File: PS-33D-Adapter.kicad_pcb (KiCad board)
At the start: 2 copper layers, 19.1 x 10.2 mm, 8 parts, among them J1 CONN_05, J2 Conn_02x04_Counter_Clockwise, Q1 MOSFET-NCH-BSS138, Q2 MOSFET-NCH-BSS138

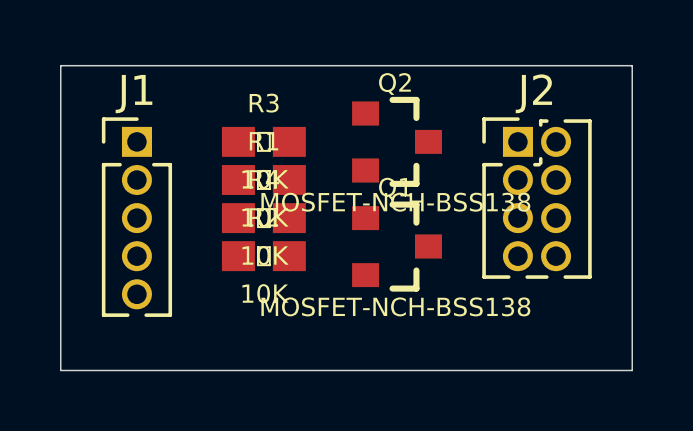
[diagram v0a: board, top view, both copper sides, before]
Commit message: feat: update pcb
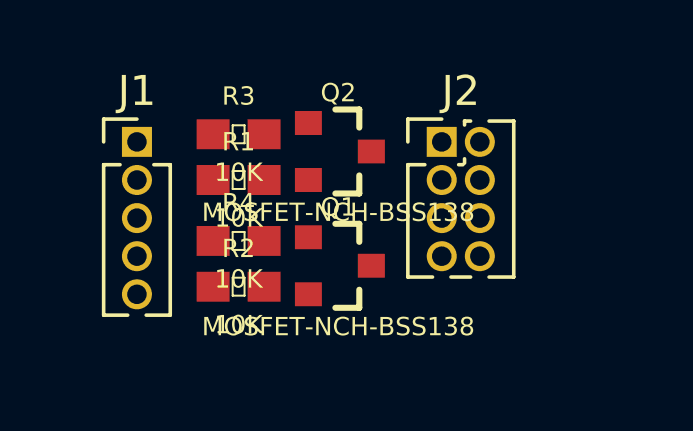
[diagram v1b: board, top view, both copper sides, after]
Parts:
- moved J2 2.54 mm to (157.5, 78.7)
- moved Q1 2.01 mm to (154.0, 82.9)
- moved Q2 1.93 mm to (154.0, 79.1)
- moved R2 1.32 mm to (150.7, 83.6)
- moved R4 1.14 mm to (150.7, 82.0)
- moved R3 0.88 mm to (150.7, 78.5)
- moved R1 0.84 mm to (150.7, 80.0)
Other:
- board outline removed
- net class Default: clearance 0.254 -> 0.15; trace_width 0.254 -> 0.25; via_dia 0.762 -> 0.6; via_drill 0.381 -> 0.3
- rule trace_clearance: 0.254 -> 0.15
- rule trace_min: 0.1524 -> 0.16
- rule via_min_drill: 0.254 -> 0.3
- rule via_min_size: 0.508 -> 0.6
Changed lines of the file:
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@@
   (general
     (thickness 1.6)
-    (drawings 4)
+    (drawings 0)
     (tracks 0)
     (zones 0)
@@
   )
   (setup
-    (last_trace_width 0.254)
-    (trace_clearance 0.254)
+    (last_trace_width 0.25)
+    (trace_clearance 0.15)
     (zone_clearance 0.508)
     (zone_45_only no)
-    (trace_min 0.1524)
-    (via_size 0.762)
-    (via_drill 0.381)
-    (via_min_size 0.508)
-    (via_min_drill 0.254)
+    (trace_min 0.16)
+    (via_size 0.6)
+    (via_drill 0.3)
+    (via_min_size 0.6)
+    (via_min_drill 0.3)
     (uvia_size 0.762)
     (uvia_drill 0.381)
@@
   (net 7 SCL)
   (net_class Default "This is the default net class."
-    (clearance 0.254)
-    (trace_width 0.254)
-    (via_dia 0.762)
-    (via_drill 0.381)
+    (clearance 0.15)
+    (trace_width 0.25)
+    (via_dia 0.6)
+    (via_drill 0.3)
     (uvia_dia 0.762)
     (uvia_drill 0.381)
@@
   )
   (module Connector_PinHeader_1.27mm:PinHeader_2x04_P1.27mm_Vertical (layer F.Cu)
-    (at 160.02 78.74)
+    (at 157.48 78.74)
     (descr "Through hole straight pin header, 2x04, 1.27mm pitch, double rows")
     (tags "Through hole pin header THT 2x04 1.27mm double row")
@@
   )
   (module Silicon-Standard:SOT23-3 (layer F.Cu)
-    (at 155.93822 82.22996 270)
+    (at 154.03322 82.87004 270)
     (descr SOT23-3)
     (tags SOT23-3)
@@
   )
   (module Silicon-Standard:SOT23-3 (layer F.Cu)
-    (at 155.93822 78.74 270)
+    (at 154.03322 79.06004 270)
     (descr SOT23-3)
     (tags SOT23-3)
@@
   )
   (module Resistors:0603 (layer F.Cu)
-    (at 151.55164 80.01)
+    (at 150.70836 80.01)
     (descr "GENERIC 1608 (0603) PACKAGE")
     (tags "GENERIC 1608 (0603) PACKAGE")
@@
   )
   (module Resistors:0603 (layer F.Cu)
-    (at 151.55164 82.55)
+    (at 150.70836 83.566)
     (descr "GENERIC 1608 (0603) PACKAGE")
     (tags "GENERIC 1608 (0603) PACKAGE")
@@
   )
   (module Resistors:0603 (layer F.Cu)
-    (at 151.55164 78.74)
+    (at 150.70836 78.486)
     (descr "GENERIC 1608 (0603) PACKAGE")
     (tags "GENERIC 1608 (0603) PACKAGE")
@@
   )
   (module Resistors:0603 (layer F.Cu)
-    (at 151.55164 81.28)
+    (at 150.70836 82.042)
     (descr "GENERIC 1608 (0603) PACKAGE")
     (tags "GENERIC 1608 (0603) PACKAGE")
@@
       (net 2 5V) (solder_mask_margin 0.1016))
   )
-  (gr_line (start 144.78 86.36) (end 144.78 76.2) (layer Edge.Cuts) (width 0.05))
-  (gr_line (start 163.83 86.36) (end 144.78 86.36) (layer Edge.Cuts) (width 0.05))
-  (gr_line (start 163.83 76.2) (end 163.83 86.36) (layer Edge.Cuts) (width 0.05))
-  (gr_line (start 144.78 76.2) (end 163.83 76.2) (layer Edge.Cuts) (width 0.05))
 )

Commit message: feat: arrange parts
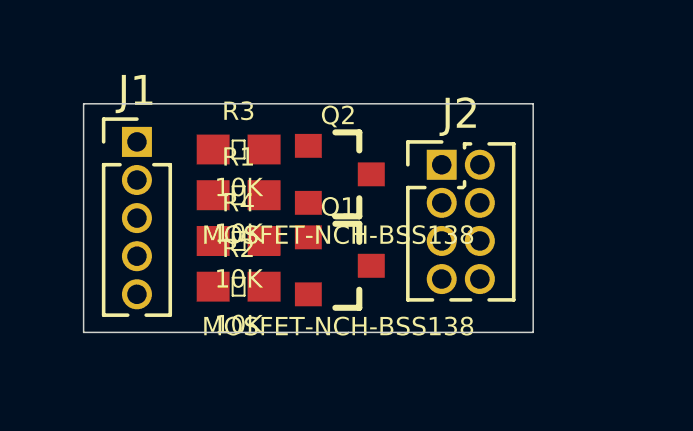
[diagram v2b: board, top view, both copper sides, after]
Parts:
- moved J2 0.76 mm to (157.5, 79.5)
- moved Q2 0.76 mm to (154.0, 79.8)
- moved R1 0.51 mm to (150.7, 80.5)
- moved R3 0.51 mm to (150.7, 79.0)
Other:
- board outline added: 15 x 7.6 mm
